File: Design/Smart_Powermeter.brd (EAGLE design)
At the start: 92 x 87 mm, 66 parts, among them IC1 AMS1117-3.3, IC3 ESP32-S2-MINI-1-N4R2, J1 AUDIO_JACK_TRRSSMD_RA, J2 AUDIO_JACK_TRRSSMD_RA, J3 AUDIO_JACK_TRRSSMD_RA, J4 AUDIO_JACK_TRRSSMD_RA, J5 AUDIO_JACK_TRRSSMD_RA, J6 AUDIO_JACK_TRRSSMD_RA, J8 USB-C, Q1 IRLML0100

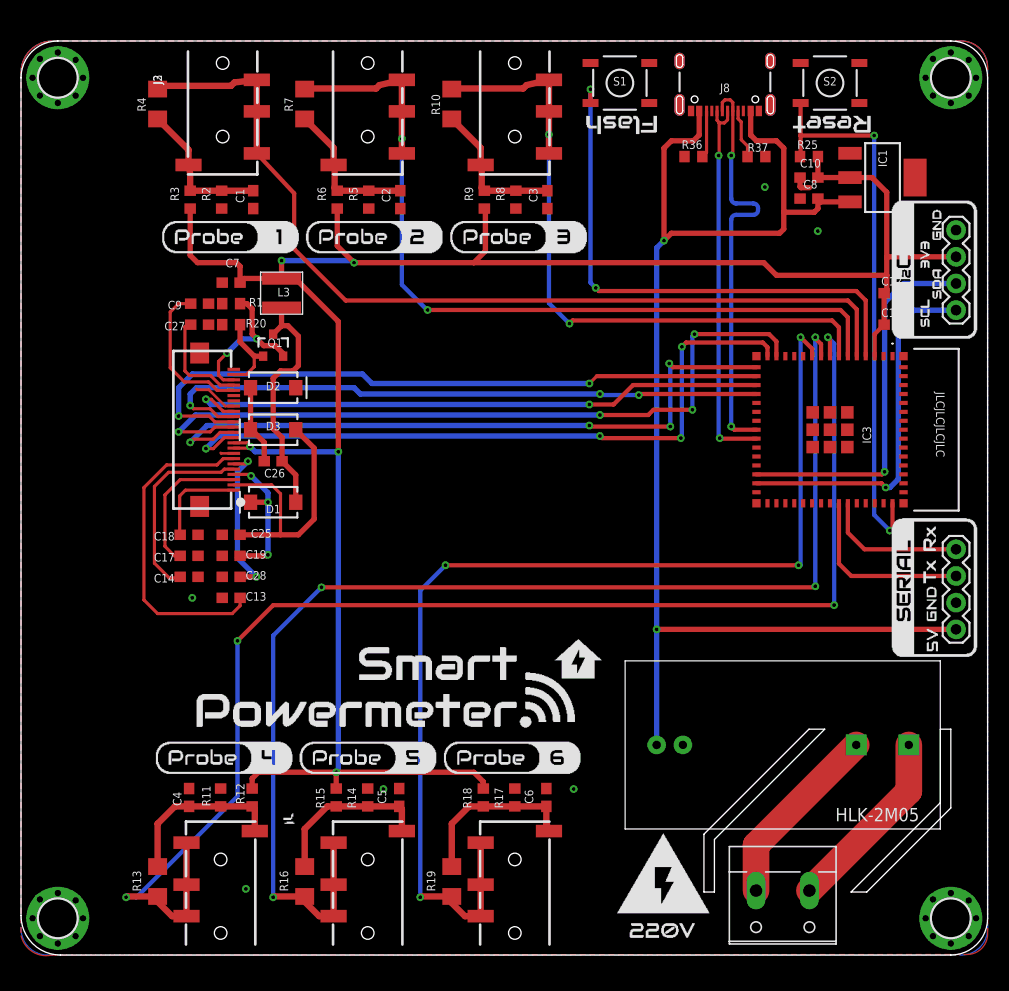
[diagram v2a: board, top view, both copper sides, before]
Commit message: First draft for the Pro version
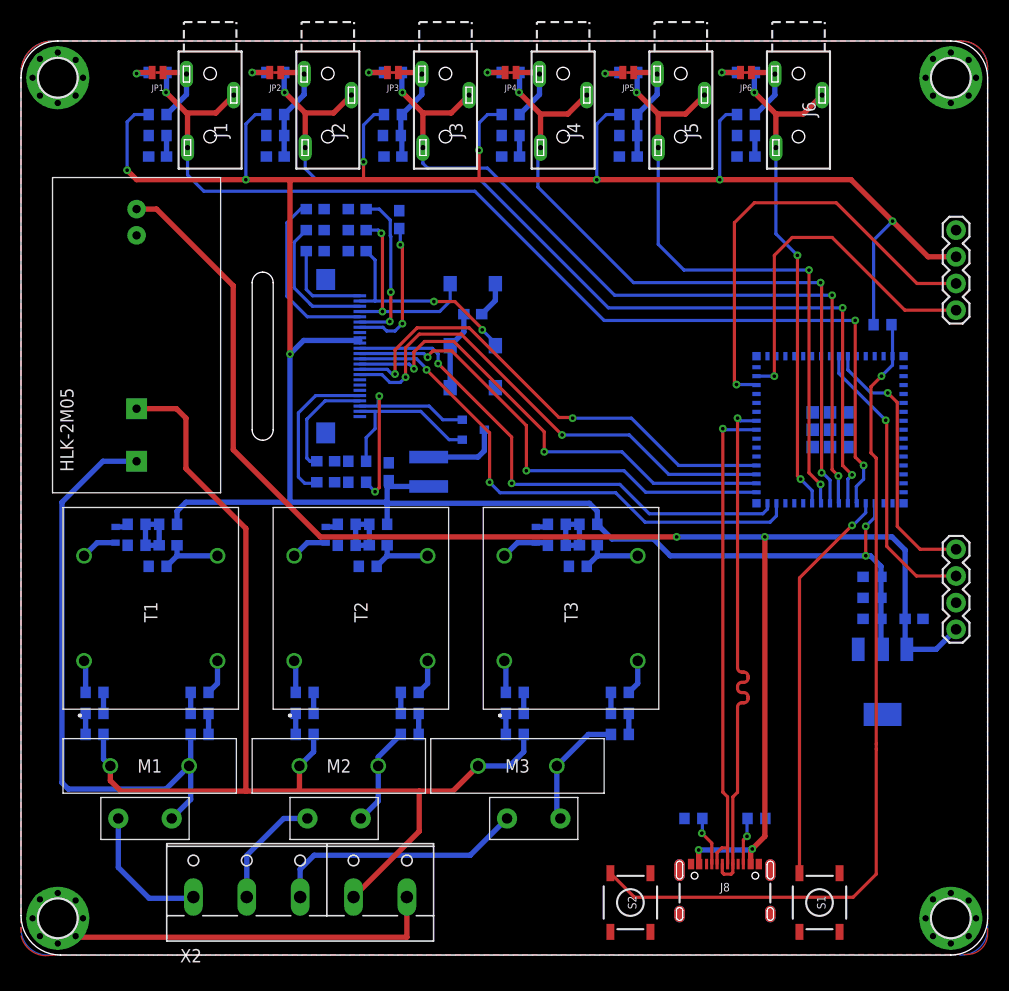
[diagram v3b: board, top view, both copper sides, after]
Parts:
- removed X1: (no value), con-wago-508:W237-132
- added C16, C20, C21: 10u/6V, rcl:C0603
- added D4, D5, D7: ESD5Z3.3T1G, microbuilder:SOD-523
- added F1, F2, F3: 1A x 250V, OpenEnergyMonitor:FUSE
- added JP1, JP2, JP3, JP4, JP5, JP6: JUMPER-SMT_2_NC_TRACE_NO-SILK, SparkFun-Jumpers:SMT-JUMPER_2_NC_TRACE_NO-SILK
- added M1, M2, M3: 275VAC, OpenEnergyMonitor:MOV
- added R21, R22, R23, R24, R26, R27, R28, R32, R33, R34, R35, R38, R39, R40, R48, R49, R50, R51, R52, R53, R54: 10k, rcl:R0603
- added R29, R41, R55: 180k, rcl:R0603
- added R30, R42, R56: 33k, rcl:R0603
- added R31, R43, R57: 1k, rcl:R0603
- added T1, T2, T3: ZMPT101B, OpenEnergyMonitor:ZMPT101B
- added X2: (no value), con-wago-508:W237-5P
- J1, J2, J3, J4, J5, J6: value AUDIO_JACK_TRRSSMD_RA -> AUDIO_JACK_MONO_3.5_3P; device SparkFun-Connectors:AUDIO_JACK_3.5MM_TRRS_SMD_RA -> SpaceDIY_connectors:HC-PJ-320A-3P-D
- R10, R13, R16, R19, R4, R7: device rcl:R1206 -> rcl:R0603
- moved J4 91.5 mm to (51.6, 86.0), turned to 180 degrees
- moved J5 90.5 mm to (62.8, 86.0), turned to 180 degrees
- moved J6 89.7 mm to (74.0, 86.0), turned to 180 degrees
- moved R13 84.0 mm to (46.6, 84.0), flipped to the bottom, turned to 0 degrees
- moved R16 82.9 mm to (57.8, 84.0), flipped to the bottom, turned to 0 degrees
- moved R19 81.9 mm to (69.0, 84.0), flipped to the bottom, turned to 0 degrees
- moved S1 80.3 mm to (76.0, 5.00), turned to 270 degrees
- moved S2 80.3 mm to (58.0, 5.00), turned to 270 degrees
- moved J8 71.0 mm to (67.0, 9.00), turned to 0 degrees
- moved R15 70.7 mm to (57.8, 80.0), flipped to the bottom, turned to 0 degrees
- moved U$2 70.3 mm to (19.0, 44.0), turned to 90 degrees
- moved R18 69.6 mm to (69.0, 80.0), flipped to the bottom, turned to 0 degrees
- moved R12 69.5 mm to (46.6, 80.0), flipped to the bottom, turned to 0 degrees
- moved R11 68.8 mm to (46.6, 78.0), flipped to the bottom, turned to 180 degrees
- moved C4 68.2 mm to (46.6, 76.0), flipped to the bottom, turned to 0 degrees
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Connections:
- removed net VG0: C1.1, J1.EARTH, R2.2, R3.1, R4.1
- new net L1: F1.IN, M1.1, R48.1, U$2.AC1
- new net L2: F2.IN, M2.1, R21.1
- new net L3: F3.IN, M3.1, R32.1
- new net N$10: R23.2, T2.2
- new net N$18: C20.1, R28.1, T2.3
- new net N$19: C20.2, R29.1, R30.2, R31.2
- new net N$20: R32.2, R33.1
- new net N$21: R33.2, R34.1
- new net N$22: R35.1, T3.1
- new net N$23: R35.2, R38.1
- new net N$24: R38.2, R39.1
- new net N$25: R48.2, R49.1
- new net N$26: R34.2, T3.2
- new net N$27: C21.1, R40.1, T3.3
- new net N$28: C21.2, R41.1, R42.2, R43.2
- new net N$29: JP2.2, R7.2
- new net N$3: F2.OUT, X2.2
- new net N$30: JP3.2, R10.2
- new net N$33: JP4.2, R13.2
- new net N$34: JP5.2, R16.2
- new net N$35: JP6.2, R19.2
- new net N$36: R49.2, R50.1
- new net N$37: R51.1, T1.1
- new net N$38: R51.2, R52.1
- new net N$39: R52.2, R53.1
- new net N$4: F3.OUT, X2.3
- new net N$40: R50.2, T1.2
- new net N$41: C16.1, R54.1, T1.3
- new net N$44: C16.2, R55.1, R56.2, R57.2
- new net N$5: R21.2, R22.1
- new net N$6: R22.2, R23.1
- new net N$7: R24.1, T2.1
- new net N$8: R24.2, R26.1
- new net N$9: R26.2, R27.1
- new net NEUTRAL: M1.2, M2.2, M3.2, R27.2, R39.2, R53.2, U$2.AC2, X2.4
- new net V1: D4.K, R57.1
- new net V2: D5.K, R31.1
- new net V3: D7.K, R43.1
- new net VG6: C6.1, J6.1, JP6.1, R17.2, R18.1
- net 3.3V: now also R29.2, R41.2, R55.2
- net GND: now also D4.A, D5.A, D7.A, R28.2, R30.1, R40.2, R42.1, R54.2, R56.1, T1.4, T2.4, T3.4, X2.5
- net M1: now also J1.2, J1.3, R4.1; no longer J1.RING1, J1.RING2, J1.TIP, R4.2
- net M2: now also J2.2, J2.3, R7.1; no longer J2.RING1, J2.RING2, J2.TIP, R7.2
- net M3: now also J3.2, J3.3, R10.1; no longer J3.RING1, J3.RING2, J3.TIP, R10.2
- net M4: now also J4.2, J4.3, R13.1; no longer J4.RING1, J4.RING2, J4.TIP, R13.2
- net M5: now also J5.2, J5.3, R16.1; no longer J5.RING1, J5.RING2, J5.TIP, R16.2
- net M6: now also J6.2, J6.3, R19.1; no longer J6.RING1, J6.RING2, J6.TIP, R19.2
- net N$1: now also JP1.2, R4.2; no longer U$2.AC2, X1.2
- net N$2: now also F1.OUT, X2.1; no longer U$2.AC1, X1.1
- net VG1: now also C1.1, J1.1, JP1.1, R2.2, R3.1; no longer C2.1, J2.EARTH, R5.2, R6.1, R7.1
- net VG2: now also C2.1, J2.1, JP2.1, R5.2, R6.1; no longer C3.1, J3.EARTH, R10.1, R8.2, R9.1
- net VG3: now also C3.1, J3.1, JP3.1, R8.2, R9.1; no longer C4.1, J4.EARTH, R11.2, R12.1, R13.1
- net VG4: now also C4.1, J4.1, JP4.1, R11.2, R12.1; no longer C5.1, J5.EARTH, R14.2, R15.1, R16.1
- net VG5: now also C5.1, J5.1, JP5.1, R14.2, R15.1; no longer C6.1, J6.EARTH, R17.2, R18.1, R19.1
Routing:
- net 3.3V: track 206.4 -> 325.6 mm, vias 5 -> 10
- net NEUTRAL: track 0.00 -> 109.2 mm
- net M4: track 129.1 -> 69.1 mm, vias 4 -> 3
- net L1: track 0.00 -> 57.6 mm
- net M5: track 118.0 -> 60.4 mm, vias 4 -> 3
- net M6: track 104.3 -> 48.4 mm, vias 4 -> 3
- net GND: track 7.30 -> 49.6 mm, vias 6 -> 0
- net RST: track 53.0 -> 80.6 mm, vias 2 -> 1
- net N$4: track 0.00 -> 24.3 mm
- net 5V: track 124.8 -> 148.4 mm, vias 2 -> 4
- net SPI_CS: track 72.0 -> 50.4 mm, vias 4 -> 2
- net SPI_CLK: track 65.4 -> 46.3 mm, vias 4 -> 2
- net SPI_MOSI: track 67.0 -> 49.2 mm, vias 4 -> 2
- net SPI_MISO: track 64.4 -> 46.7 mm
- net N$12: track 31.1 -> 13.7 mm, vias 0 -> 2
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
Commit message: Updated design files
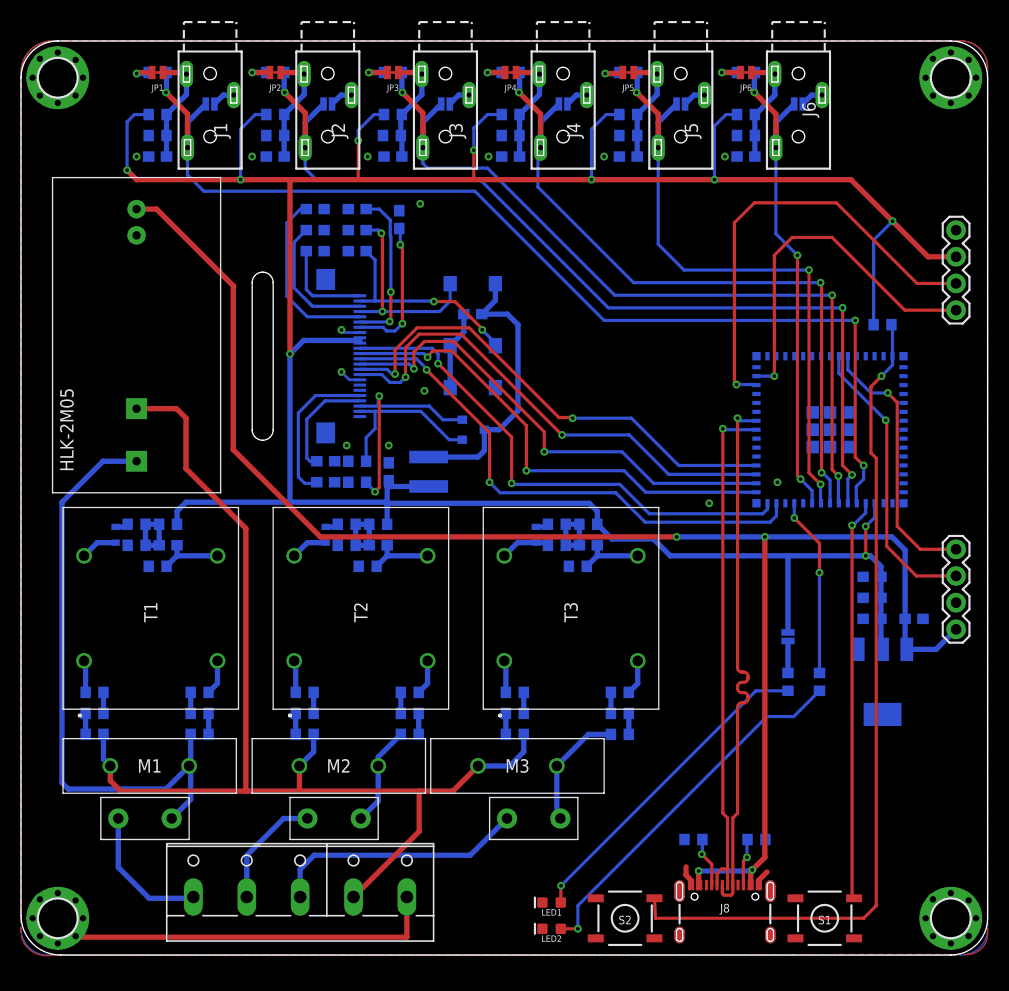
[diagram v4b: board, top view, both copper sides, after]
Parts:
- added JP10, JP11, JP12, JP7, JP8, JP9: JUMPER-SMT_2_NO_NO-SILK, SparkFun-Jumpers:SMT-JUMPER_2_NO_NO-SILK
- added JP13: JUMPER-SMT_2_NC_PASTE_NO-SILK, SparkFun-Jumpers:SMT-JUMPER_2_NC_PASTE_NO-SILK
- added LED1: GREEN, SparkFun-LED:LED-0603
- added LED2: BLUE, SparkFun-LED:LED-0603
- added R44: 470, rcl:R0603
- added R45: 330, rcl:R0603
- moved J8 2.00 mm to (67.0, 7.00)
- moved R36 2.00 mm to (70.0, 11.0)
- moved R37 2.00 mm to (64.0, 11.0)
- moved S1 1.58 mm to (76.5, 3.50), turned to 180 degrees
- moved S2 1.58 mm to (57.5, 3.50), turned to 180 degrees
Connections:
- new net LED: IC3.12, R45.2
- new net N$42: LED1.A, R44.1
- new net N$43: JP13.2, R44.2
- new net N$45: LED2.A, R45.1
- new net N$46: J1.2, JP8.2
- new net N$47: J2.2, JP7.2
- new net N$48: J3.2, JP9.2
- new net N$49: J4.2, JP10.2
- new net N$50: J5.2, JP11.2
- new net N$51: J6.2, JP12.2
- net 3.3V: now also JP13.1
- net GND: now also LED1.C, LED2.C
- net M1: now also JP8.1; no longer J1.2
- net M2: now also JP7.1; no longer J2.2
- net M3: now also JP9.1; no longer J3.2
- net M4: now also JP10.1; no longer J4.2
- net M5: now also JP11.1; no longer J5.2
- net M6: now also JP12.1; no longer J6.2
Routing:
- net N$45: track 0.00 -> 35.3 mm, vias 0 -> 1
- net N$42: track 0.00 -> 30.9 mm, vias 0 -> 1
- net LED: track 0.00 -> 17.1 mm, vias 0 -> 2
- net N$17: track 11.0 -> 27.0 mm
- net GND: track 49.6 -> 57.0 mm, vias 0 -> 14
- net N$43: track 0.00 -> 3.04 mm
- net N$49: track 0.00 -> 2.20 mm
- net N$48: track 0.00 -> 2.20 mm
- net N$47: track 0.00 -> 2.20 mm
- net N$46: track 0.00 -> 2.20 mm
- net N$51: track 0.00 -> 2.20 mm
- net N$50: track 0.00 -> 2.20 mm
- net VG6: track 8.96 -> 11.0 mm
- net VG4: track 8.93 -> 10.9 mm
- net VG1: track 8.93 -> 10.9 mm
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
